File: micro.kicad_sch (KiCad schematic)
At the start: 35 parts, among them J7 USB_C_Receptacle_USB2.0_16P, J8 Conn_01x04_Pin, J9 Conn_01x06_Pin, SW2 SW_Push, U4 STM32F411RETx, U5 TME-0505S, U6 ADUM3160, Y2 8M

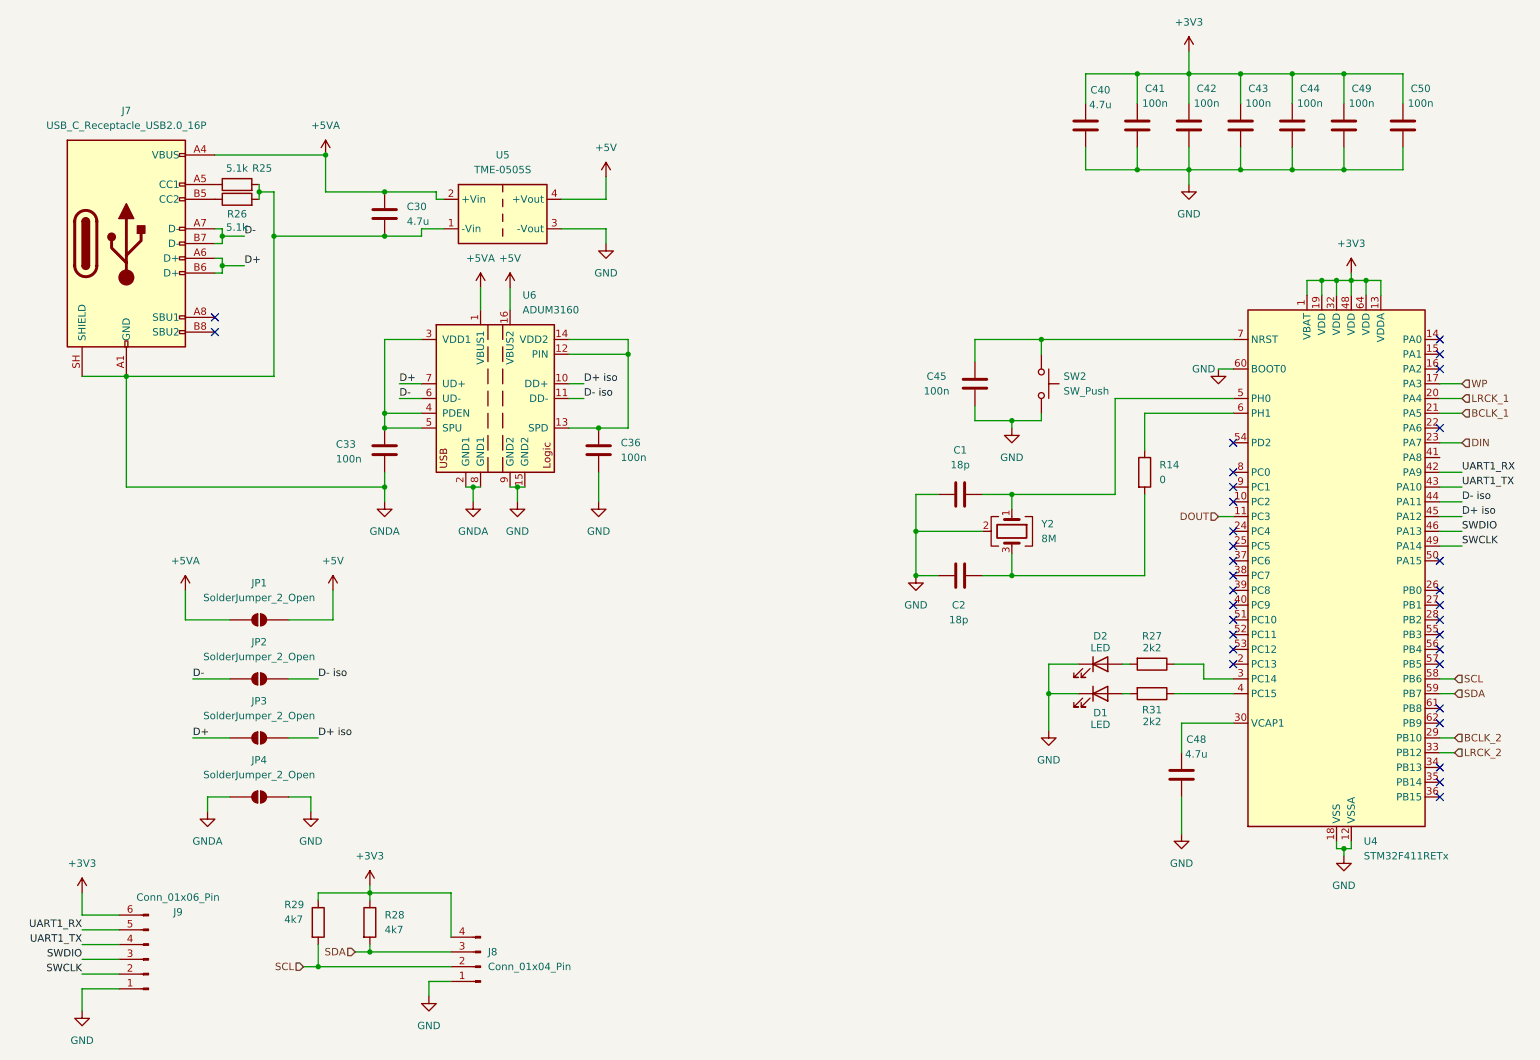
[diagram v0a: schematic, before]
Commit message: pulito lo schematico e fatto dei check
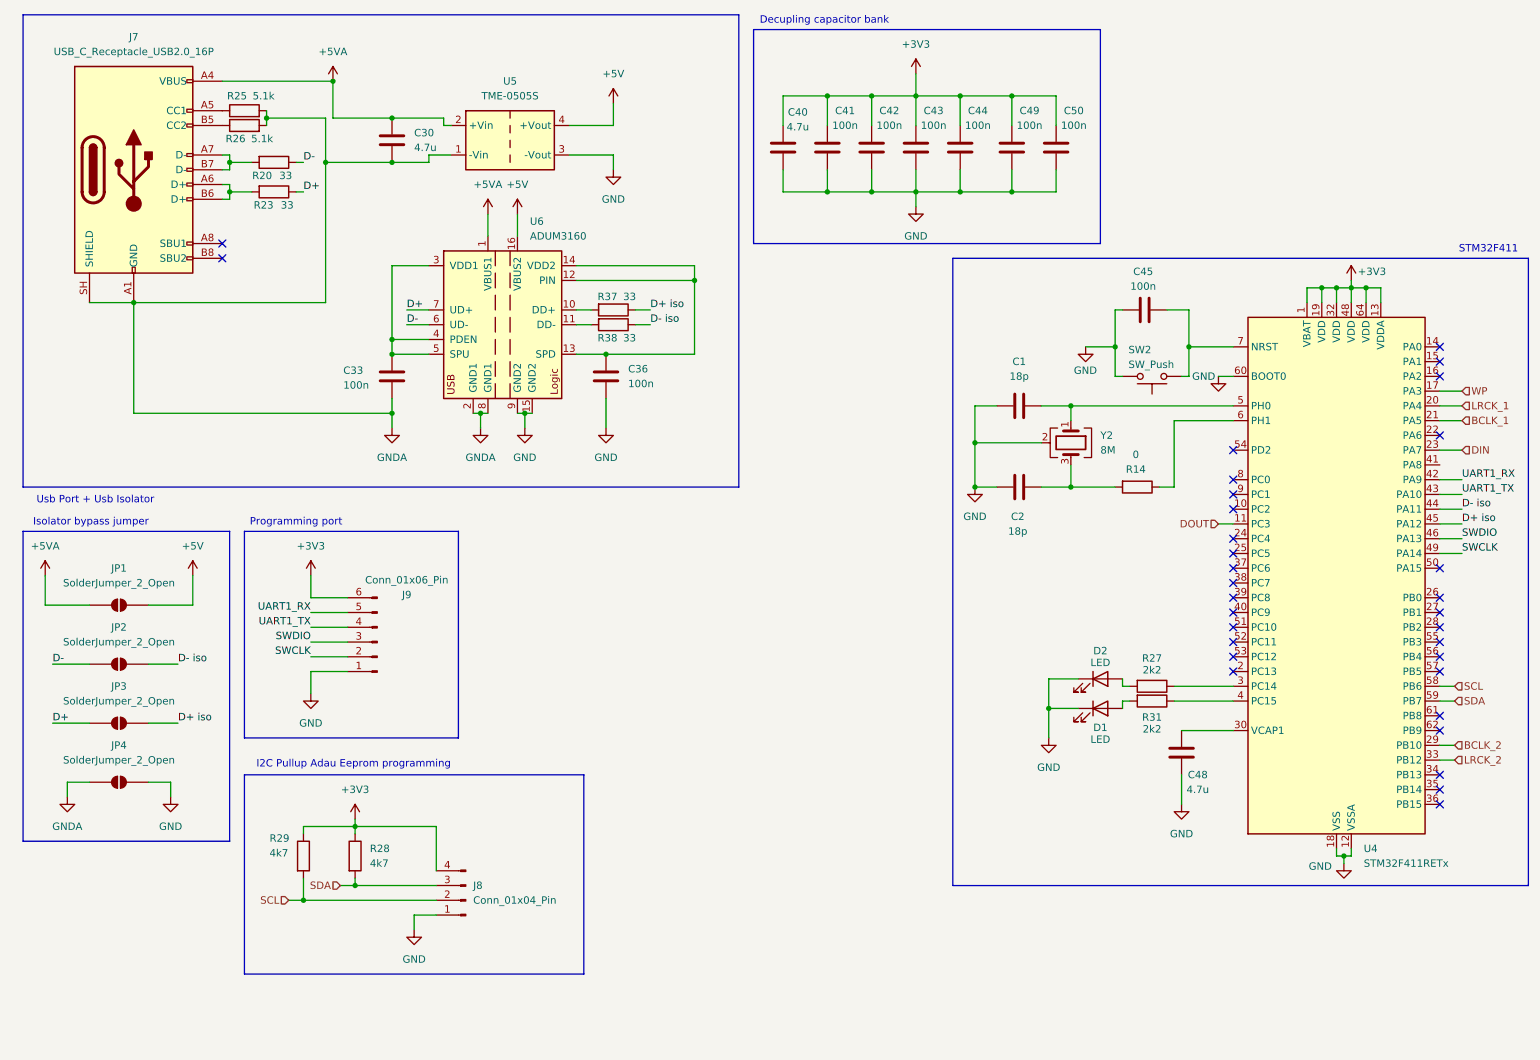
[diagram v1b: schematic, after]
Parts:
- added R20, R23, R37, R38: 33, Resistor_SMD:R_0603_1608Metric, symbol Device:R
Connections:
- net D+: now also R23.1; no longer J7.A6 (D+), J7.B6 (D+)
- net D+ iso: now also R37.1; no longer U6.10 (DD+)
- net D-: now also R20.1; no longer J7.A7 (D-), J7.B7 (D-)
- net D- iso: now also R38.1; no longer U6.11 (DD-)
- new net: R38.2, U6.11 (DD-)
- new net: J7.A6 (D+), J7.B6 (D+), R23.2
- new net: J7.A7 (D-), J7.B7 (D-), R20.2
- new net: R37.2, U6.10 (DD+)
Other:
- note added: "Decupling capacitor bank"
- note added: "I2C Pullup Adau Eeprom programming"
- note added: "Isolator bypass jumper"
- note added: "Programming port"
- note added: "STM32F411"
- note added: "Usb Port + Usb Isolator"
- moved on the sheet: C1, C2, C30, C33, C36, C40, C41, C42, C43, C44, C45, C48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
